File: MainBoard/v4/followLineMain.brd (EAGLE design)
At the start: 95 x 53.1 mm, 32 parts, among them IC1 L298, J1 DCJ0202, X1 332-02, X2 332-02

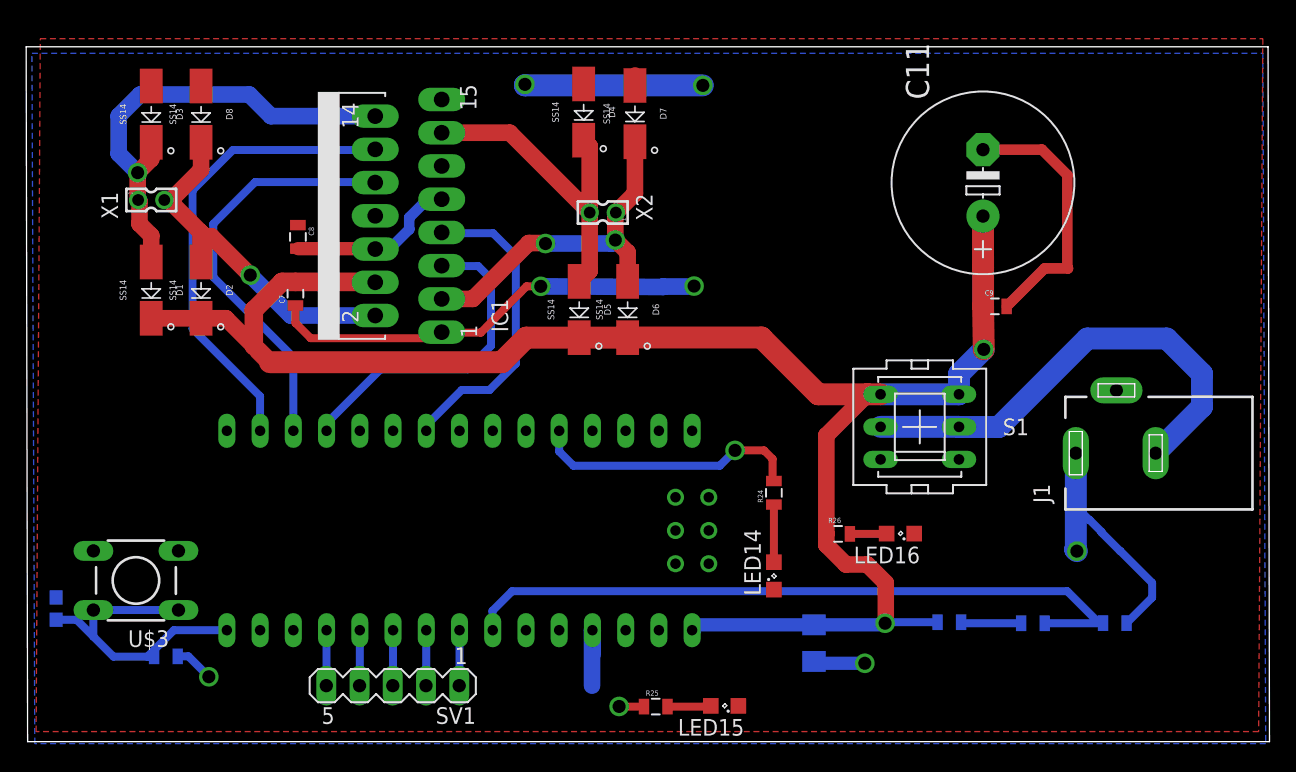
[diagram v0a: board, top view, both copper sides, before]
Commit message: nothing changed...
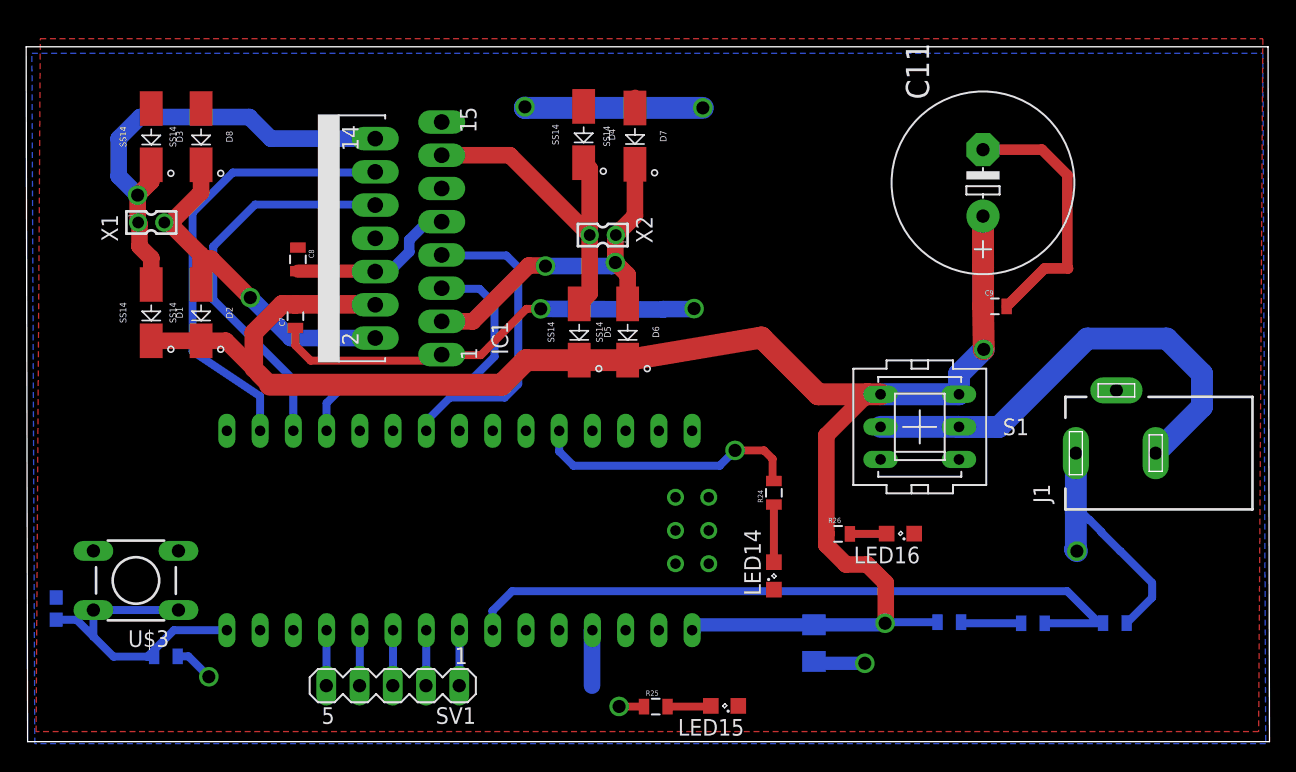
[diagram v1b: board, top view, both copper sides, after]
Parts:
- moved X1 1.72 mm to (9.56, 39.7)
- moved C7 1.72 mm to (20.6, 32.5)
- moved C8 1.72 mm to (20.8, 36.8)
- moved D1 1.72 mm to (9.56, 32.8)
- moved D2 1.72 mm to (13.4, 32.8)
- moved D3 1.72 mm to (9.56, 46.2)
- moved D4 1.72 mm to (42.6, 46.4)
- moved D5 1.72 mm to (42.3, 31.3)
- moved D6 1.72 mm to (46.0, 31.3)
- moved D7 1.72 mm to (46.5, 46.3)
- moved D8 1.72 mm to (13.4, 46.2)
- moved IC1 1.72 mm to (24.1, 38.5)
- moved X2 1.72 mm to (44.1, 38.7)
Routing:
- net N$14: track 1.83 -> 0.00 mm
- net PWM3: track 32.1 -> 30.3 mm
- net PWM4: track 35.8 -> 34.7 mm
